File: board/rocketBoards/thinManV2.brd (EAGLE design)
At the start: 45 x 18 mm, 48 parts, among them J1 47346-0001

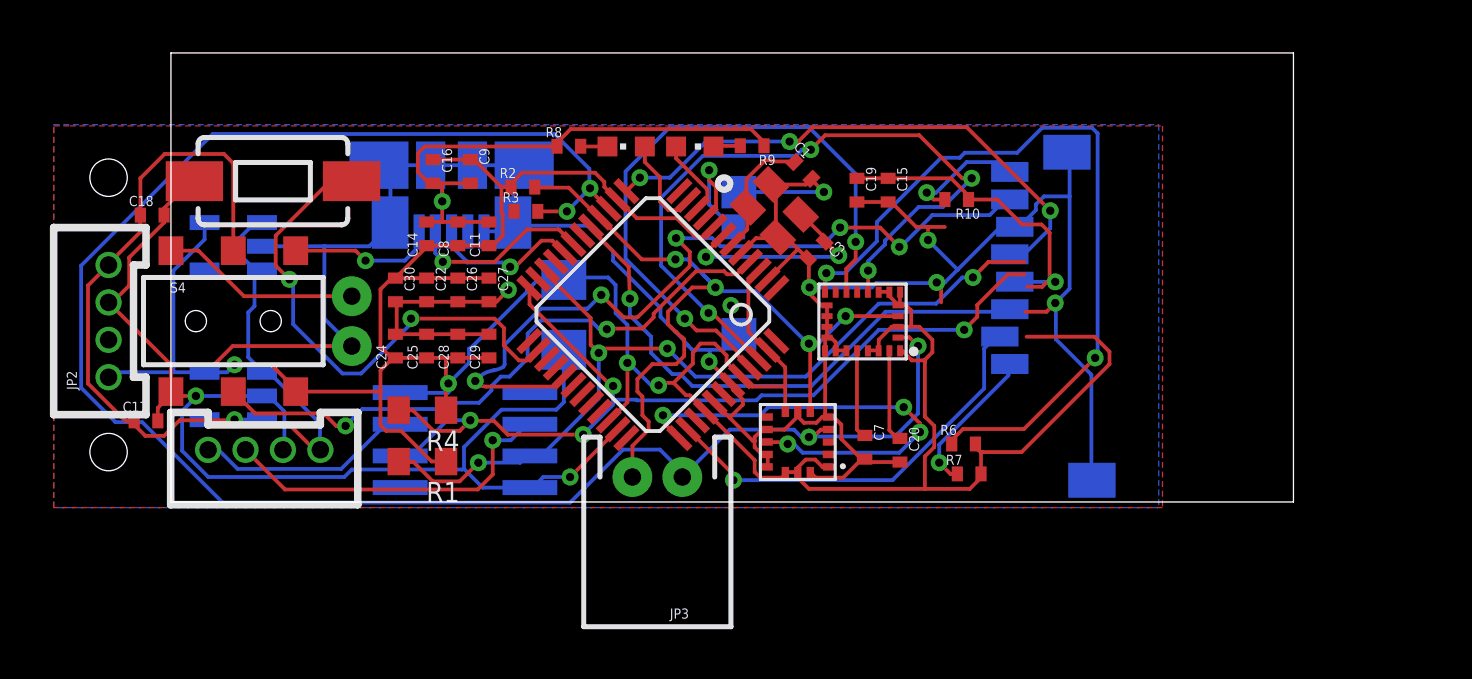
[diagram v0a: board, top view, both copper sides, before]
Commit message: thinManV2 changes
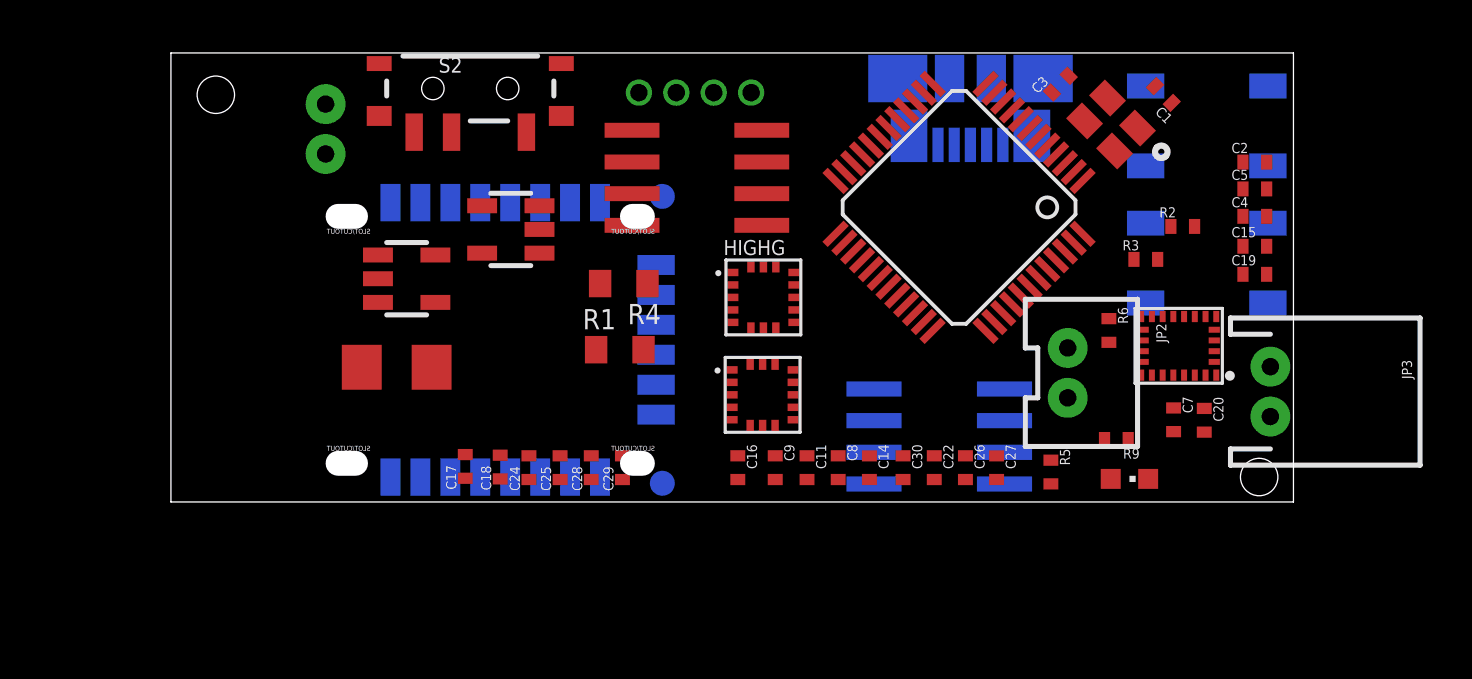
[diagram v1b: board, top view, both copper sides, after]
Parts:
- removed LED1: (no value), adafruit:CHIPLED_0603
- removed R10, R7, R8: (no value), ELL-i-Passives:R0402
- removed S1: SWITCH-MOMENTARY-2-SMD-1101NE, SparkFun-Electromechanical:TACTILE-SWITCH-1101NE
- removed S4: DPDT, SparkFun-Electromechanical:AYZ0202
- removed U$3: MICROSD-CD, Sensors:MOLEX_SD-47352-101
- added C2: 10uF, ELL-i-Passives:C0402
- added C4, C5: .1uF, ELL-i-Passives:C0402
- added D1, D2: (no value), SparkFun-LED:WS2812B
- added HIGHG: LPS331AP, Sensors:LGA-16-3X3X1
- added R5: (no value), ELL-i-Passives:R0402
- added S2: (no value), SparkFun-Electromechanical:SWITCH-SPST-SMD-A
- added U$1: RN4020, bluetooth:RN4020
- added U$7: S25FL127S, SparkFun-DigitalIC:SO08
- JP2: value (none) -> M02JST-PTH-VERT; device SparkFun-Connectors:1X04-1.5MM_JST -> SparkFun-Connectors:JST-2-PTH-VERT
- moved JP2 39.0 mm to (36.5, 5.17), turned to 270 degrees
- moved R2 26.5 mm to (40.6, 11.0)
- moved R3 24.9 mm to (39.1, 9.72)
- moved JP3 24.8 mm to (44.1, 4.42), turned to 270 degrees
- moved JP6 22.4 mm to (23.3, 16.4), flipped to the bottom, turned to 0 degrees
- moved LED2 21.9 mm to (38.4, 0.93)
- moved C22 21.6 mm to (30.6, 1.38)
- moved C26 21.6 mm to (31.9, 1.38)
- moved C27 21.6 mm to (33.1, 1.38)
- moved C30 21.6 mm to (29.4, 1.38)
- moved J1 21.1 mm to (32.0, 17.0)
- moved C14 20.1 mm to (28.0, 1.38), turned to 270 degrees
- moved R9 18.8 mm to (37.9, 2.50)
- moved C8 17.9 mm to (26.8, 1.38), turned to 270 degrees
- moved U$5 17.4 mm to (39.5, 14.9), turned to 135 degrees
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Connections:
- removed net BARO_INT2: U1.33
- removed net HIGHG_INT2: U1.36
- removed net INT2_A/G: U1.42
- removed net N$16: R7.1, U$3.1
- removed net N$19: S1.1, U1.26
- removed net N$21: R10.2, U$3.8
- new net N$6: D1.2, D2.4
- new net PIXEL: D1.4, U1.30
- new net SSP1_RST: U$7.7
- net 3.3V: now also C2.1, C4.1, C5.1, D1.1, D2.1, HIGHG.1, HIGHG.14, HIGHG.15, HIGHG.8, R5.2, U$7.8; no longer JP2.1, R10.1, R7.2, S4.6, U$3.4
- net GND: now also C2.2, C4.2, C5.2, D1.3, D2.3, HIGHG.10, HIGHG.12, HIGHG.13, HIGHG.16, HIGHG.5, HIGHG.7, JP2.2; no longer JP2.3, R8.1, S1.2, S4.4, U$3.6, U$3.G1, U$3.G2, U$3.G3, U$3.G4
- net HIGHG_INT1: now also HIGHG.11; no longer U1.32
- net I2C0_SCL: now also HIGHG.4
- net I2C0_SDA: now also HIGHG.6
- net LED_PIN2: no longer LED1.A
- net N$20: now also S2.1; no longer S4.1
- net N$4: now also R5.1, U$7.3; no longer LED1.C, R8.2
- net PIO0_1: now also JP2.1; no longer S4.5
- net SD_CD: no longer U$3.9
- net SSP1_MISO: now also U$7.2; no longer U$3.7
- net SSP1_MOSI: now also U$7.5; no longer U$3.3
- net SSP1_SCK: now also U$7.6; no longer U$3.5
- net SSP1_SSEL: now also U$7.1; no longer U$3.2
- net USB_VBUS: now also S2.3; no longer S4.3
- net VBUS: now also S2.2; no longer JP2.4, S4.2
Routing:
- net GND: track 199.8 -> 0.00 mm, vias 11 -> 0
- net 3.3V: track 148.1 -> 0.00 mm, vias 5 -> 0
- net I2C0_SCL: track 75.2 -> 0.00 mm, vias 4 -> 0
- net VBUS: track 40.9 -> 0.00 mm, vias 1 -> 0
- net I2C1_SCL: track 38.2 -> 0.00 mm, vias 4 -> 0
- net I2C1_SDA: track 35.4 -> 0.00 mm, vias 4 -> 0
- net I2C0_SDA: track 32.1 -> 0.00 mm, vias 4 -> 0
- net SSP1_MISO: track 31.7 -> 0.00 mm, vias 5 -> 0
- net N$1: track 30.9 -> 0.00 mm, vias 2 -> 0
- net DRDY_M: track 29.3 -> 0.00 mm, vias 4 -> 0
- net INT1_A/G: track 26.0 -> 0.00 mm, vias 2 -> 0
- net PIO0_1: track 25.2 -> 0.00 mm, vias 2 -> 0
- net SSP1_MOSI: track 22.3 -> 0.00 mm, vias 1 -> 0
- net SSP1_SCK: track 22.2 -> 0.00 mm, vias 3 -> 0
- net N$19: track 20.7 -> 0.00 mm, vias 2 -> 0
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- removed copper zone on layer 1, net GND
- removed copper zone on layer 16, net GND
